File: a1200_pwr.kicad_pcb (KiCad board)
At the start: 2 copper layers, 23.2 x 58.2 mm, 20 parts, among them J1 PJ-102A, J2 APWR_big, J3 APWR_small, SW1 RMS1R102M7QES, U1 LMZM23600SILR, U2 RPM5.0-6.0

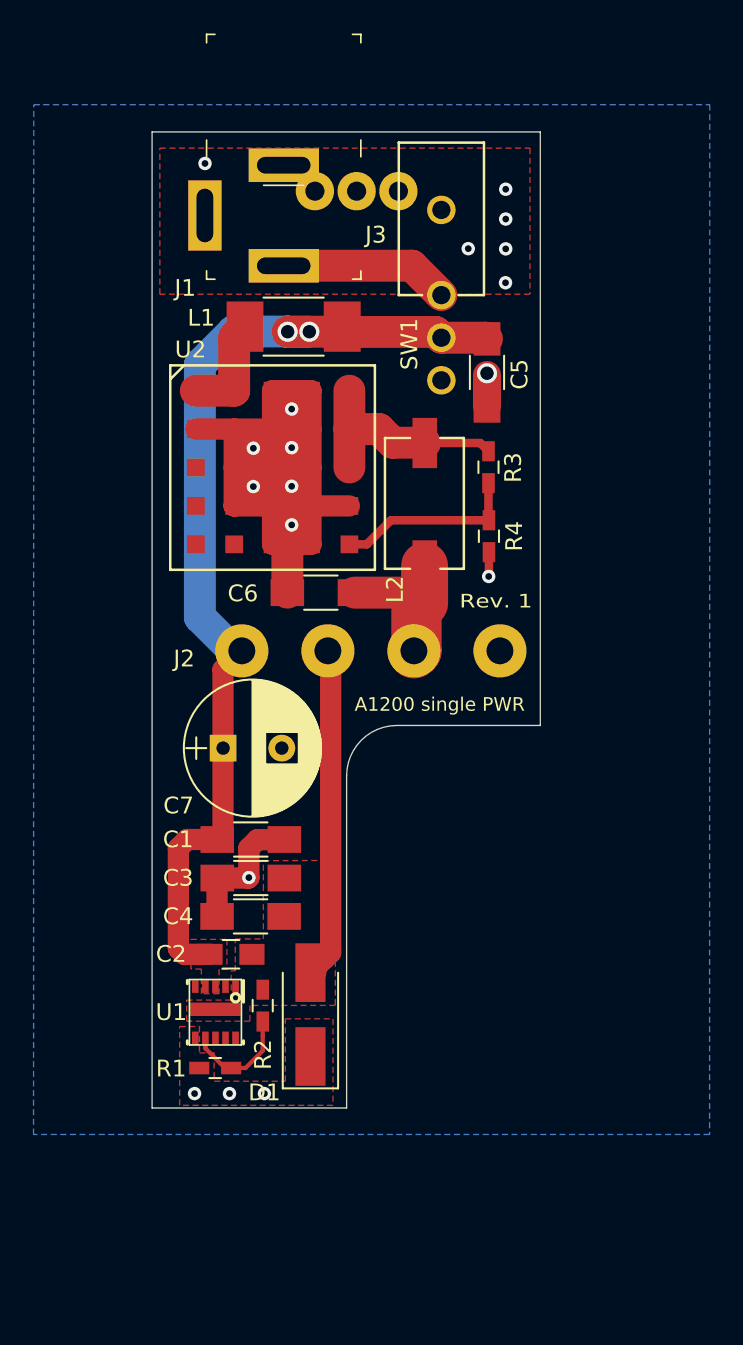
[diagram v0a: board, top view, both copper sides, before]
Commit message: Revision 2
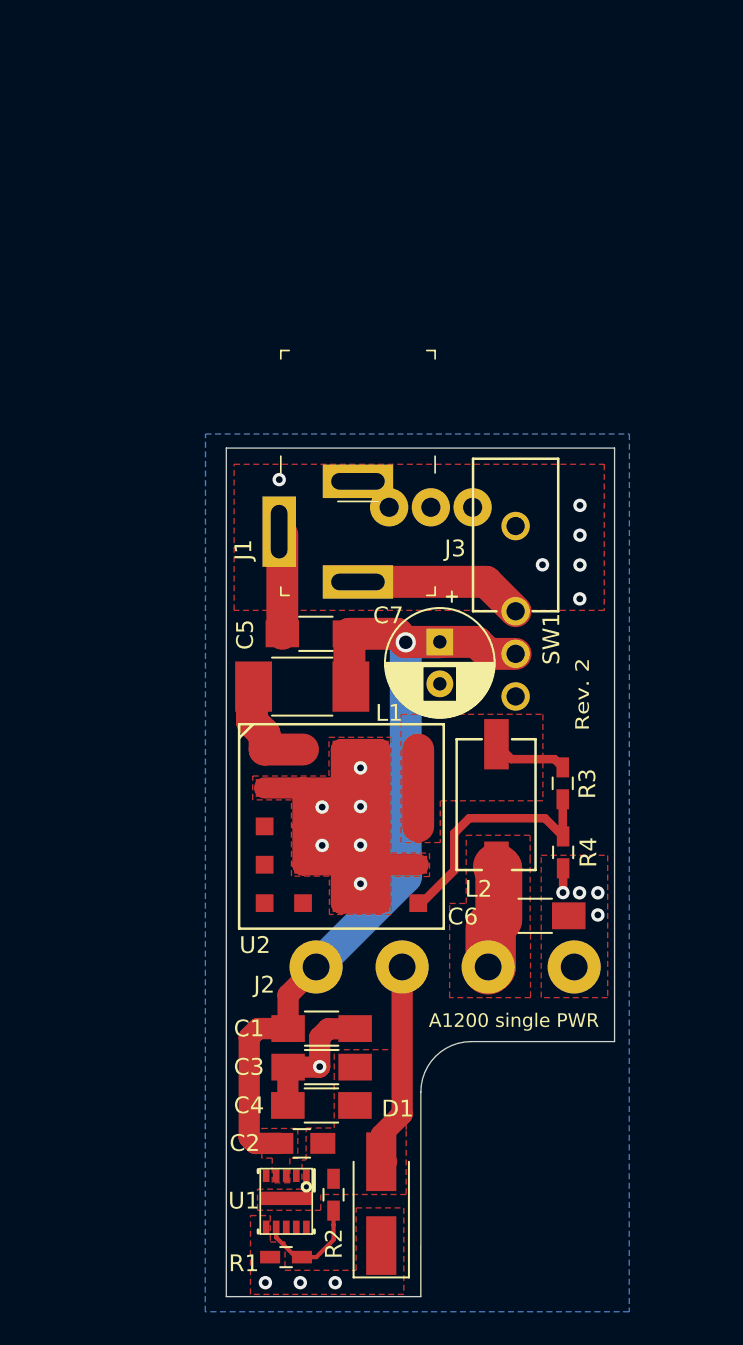
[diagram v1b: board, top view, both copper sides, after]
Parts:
- C7: footprint Capacitors_THT:CP_Radial_D8.0mm_P3.50mm -> Capacitor_THT:CP_Radial_D6.3mm_P2.50mm
- SW1: value RMS1R102M7QES -> SW_SPDT
- moved C6 23.1 mm to (156.7, 107.3), turned to 0 degrees
- moved U2 21.8 mm to (145.1, 102.1)
- moved L1 21.5 mm to (142.8, 93.7)
- moved J2 19.4 mm to (151.3, 110.4)
- moved J1 19.4 mm to (146.1, 84.4)
- moved R4 19.4 mm to (158.4, 103.6)
- moved SW1 19.4 mm to (155.5, 84.1)
- moved J3 19.4 mm to (150.5, 83.0)
- moved R3 19.4 mm to (158.3, 99.4)
- moved C5 18.6 mm to (143.6, 90.5), turned to 180 degrees
- moved L2 18.5 mm to (154.4, 100.7)
- moved C7 14.4 mm to (151.0, 91.0), turned to -90 degrees
- moved C2 12.0 mm to (142.8, 120.9)
- moved D1 12.0 mm to (147.5, 124.5)
- moved C1 12.0 mm to (144.0, 114.1)
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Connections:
- net Net-(L2-Pad2) renamed /5Vout
- SW1 pad 3: Net-(SW1-Pad3) -> unconnected-(SW1-Pad3)
- U1 pad 10: Net-(U1-Pad10) -> unconnected-(U1-Pad10)
- U1 pad 2: Net-(U1-Pad2) -> unconnected-(U1-Pad2)
- U1 pad 5: Net-(U1-Pad5) -> (no net)
- U1 pad 8: Net-(U1-Pad8) -> unconnected-(U1-Pad8)
- U1 pad 9: Net-(U1-Pad9) -> unconnected-(U1-Pad9)
- U2 pad C1: Net-(U2-PadC1) -> unconnected-(U2-PadC1)
- U2 pad D1: Net-(U2-PadD1) -> unconnected-(U2-PadD1)
- U2 pad E1: Net-(U2-PadE1) -> unconnected-(U2-PadE1)
- U2 pad E2: Net-(U2-PadE2) -> unconnected-(U2-PadE2)
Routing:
- net +12V: track 60.8 -> 52.6 mm, vias 2 -> 1
- net -12V: track 20.6 -> 12.7 mm
- net /5Vout: track 13.4 -> 9.10 mm
- net Net-(R3-Pad1): track 11.1 -> 14.7 mm
- net +5V: track 9.26 -> 5.76 mm
- net GND: track 79.1 -> 80.3 mm, vias 18 -> 20
- added copper zone on F.Cu, net +5V
- added copper zone on F.Cu, net /5Vout
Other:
- board size 23.2 x 58.2 mm -> 23.2 x 50.6 mm
- net class Default removed
- board text added: "Rev. 2"
- board text removed: "Rev. 1"
